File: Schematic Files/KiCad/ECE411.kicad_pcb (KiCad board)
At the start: 2 copper layers, 114.9 x 90.8 mm, 9 parts, among them J1-ToPump1 Conn_01x02_Female, J2-ToMoistSense1 Conn_01x02_Female, Q1 2N7002

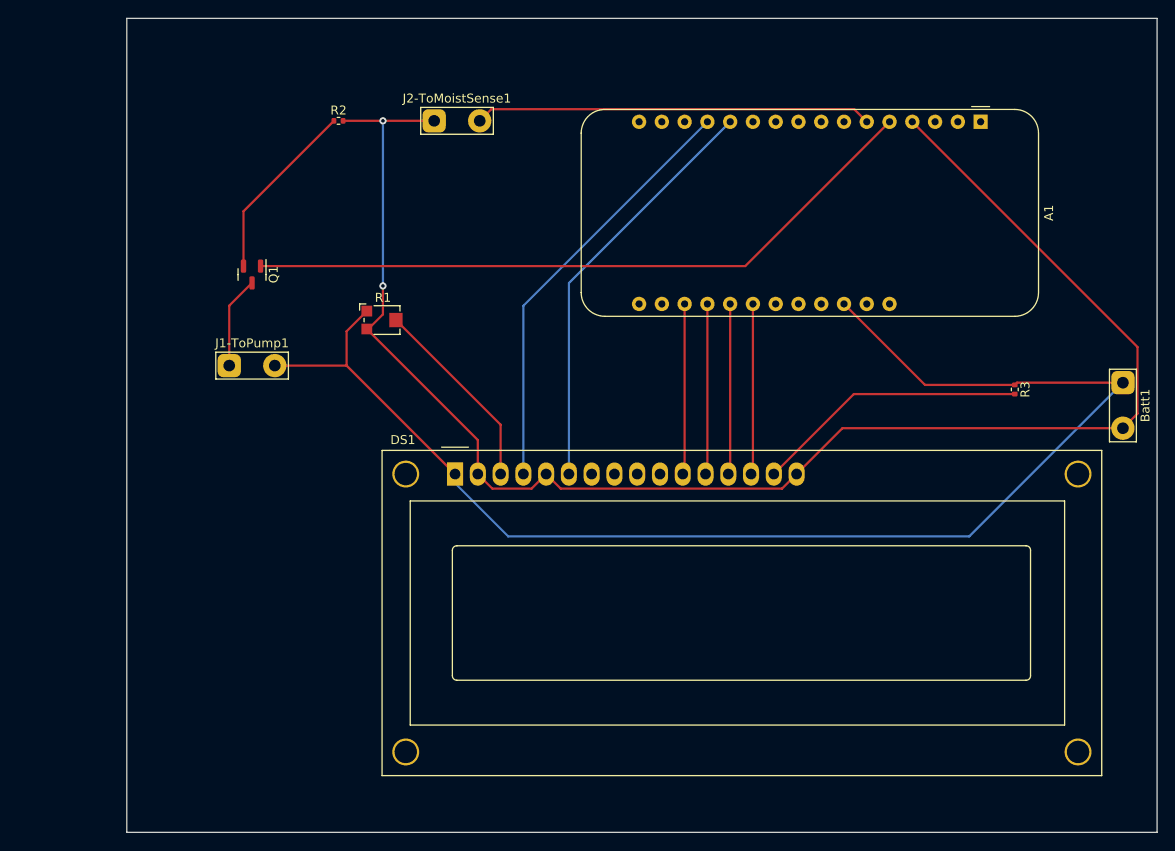
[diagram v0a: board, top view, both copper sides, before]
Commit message: Add files via upload
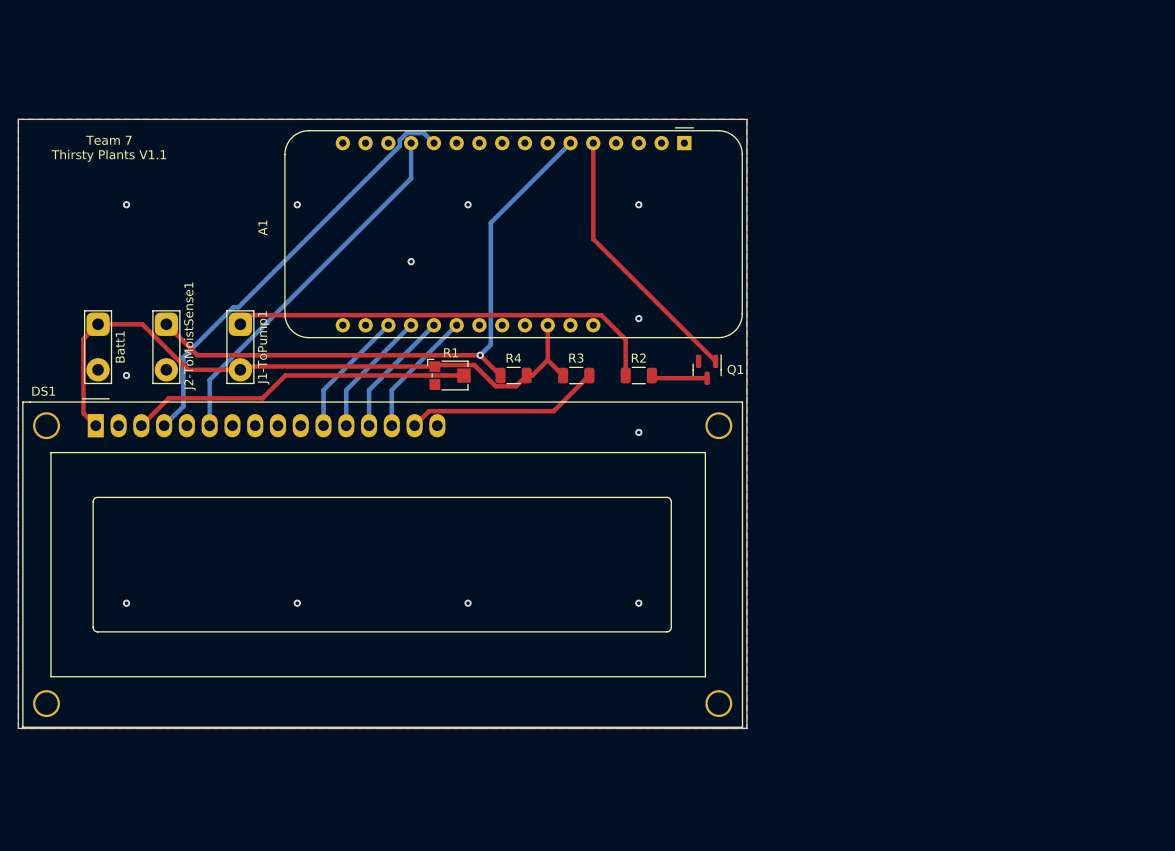
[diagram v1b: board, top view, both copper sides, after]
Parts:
- added R4: 150 Ohm, Resistor_SMD:R_1206_3216Metric, F.Cu at (162.5, 90.0)
- R1: value 10K Potentiometer -> 10K Ohm
- R2, R3: footprint Resistor_SMD:R_0402_1005Metric -> Resistor_SMD:R_1206_3216Metric
- moved Batt1 114.5 mm to (116.2, 84.3)
- moved Q1 51.9 mm to (184.1, 89.4)
- moved R3 48.9 mm to (169.5, 90.0), turned to 0 degrees
- moved R2 43.9 mm to (176.5, 90.0)
- moved DS1 40.4 mm to (115.9, 95.6)
- moved J2-ToMoistSense1 37.5 mm to (123.8, 84.3), turned to -90 degrees
- moved A1 33.1 mm to (181.6, 64.1)
- moved R1 9.79 mm to (155.5, 90.0)
- moved J1-ToPump1 4.77 mm to (132.1, 84.3), turned to -90 degrees
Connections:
- net Net-(A1-Pad26) renamed +BATT
- A1 pad 12: Net-(A1-Pad12) -> Net-(DS1-Pad4)
- A1 pad 13: Net-(A1-Pad13) -> Net-(DS1-Pad6)
- A1 pad 4: Net-(A1-Pad4) -> GND
- Batt1 pad 2: Net-(A1-Pad4) -> GND
- DS1 pad 16: Net-(A1-Pad4) -> GND
- DS1 pad 2: Net-(A1-Pad4) -> GND
- DS1 pad 4: Net-(A1-Pad13) -> Net-(DS1-Pad4)
- DS1 pad 5: Net-(A1-Pad4) -> GND
- DS1 pad 6: Net-(A1-Pad12) -> Net-(DS1-Pad6)
- J1-ToPump1 pad 1: Net-(J1-ToPump1-Pad1) -> Net-(R2-Pad1)
- J2-ToMoistSense1 pad 1: Net-(A1-Pad4) -> Net-(A1-Pad6)
- J2-ToMoistSense1 pad 2: Net-(A1-Pad6) -> GND
- Q1 pad 2: Net-(Q1-Pad2) -> GND
- Q1 pad 3: Net-(J1-ToPump1-Pad1) -> Net-(Q1-Pad3)
- R1 pad 3: Net-(A1-Pad4) -> GND
- R2 pad 1: Net-(Q1-Pad2) -> Net-(R2-Pad1)
- R2 pad 2: Net-(A1-Pad4) -> Net-(Q1-Pad3)
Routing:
- net Net-(A1-Pad4): track 177.6 -> 0.00 mm, vias 2 -> 0
- net +BATT: track 152.2 -> 73.8 mm
- net Net-(R2-Pad1): track 0.00 -> 48.5 mm
- net Net-(A1-Pad13): track 47.8 -> 0.00 mm
- net Net-(DS1-Pad4): track 0.00 -> 47.7 mm
- net Net-(A1-Pad5): track 76.8 -> 30.0 mm
- net Net-(A1-Pad12): track 46.7 -> 0.00 mm
- net Net-(DS1-Pad6): track 0.00 -> 40.8 mm
- net Net-(A1-Pad6): track 44.3 -> 67.5 mm, vias 0 -> 1
- net Net-(Q1-Pad2): track 20.4 -> 0.00 mm
- net Net-(R1-Pad2): track 22.0 -> 38.3 mm
- net Net-(J1-ToPump1-Pad1): track 10.3 -> 0.00 mm
- net Net-(R3-Pad2): track 30.6 -> 21.8 mm
- net Net-(Q1-Pad3): track 0.00 -> 6.28 mm
- net Net-(A1-Pad21): track 19.1 -> 14.2 mm
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- added copper zone on B.Cu, net GND
- added copper zone on F.Cu, net GND
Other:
- board size 114.9 x 90.8 mm -> 81.3 x 67.9 mm
- rule pad_to_mask_clearance: 0 -> 0.0508
- board text added: "Team 7 Thirsty Plants V1.1"
